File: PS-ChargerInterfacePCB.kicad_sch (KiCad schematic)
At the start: 17 parts, among them J2 LV_Elcon_Connector, J4 PeripheralCAN, J5 Estop 2, J6 Estop 3

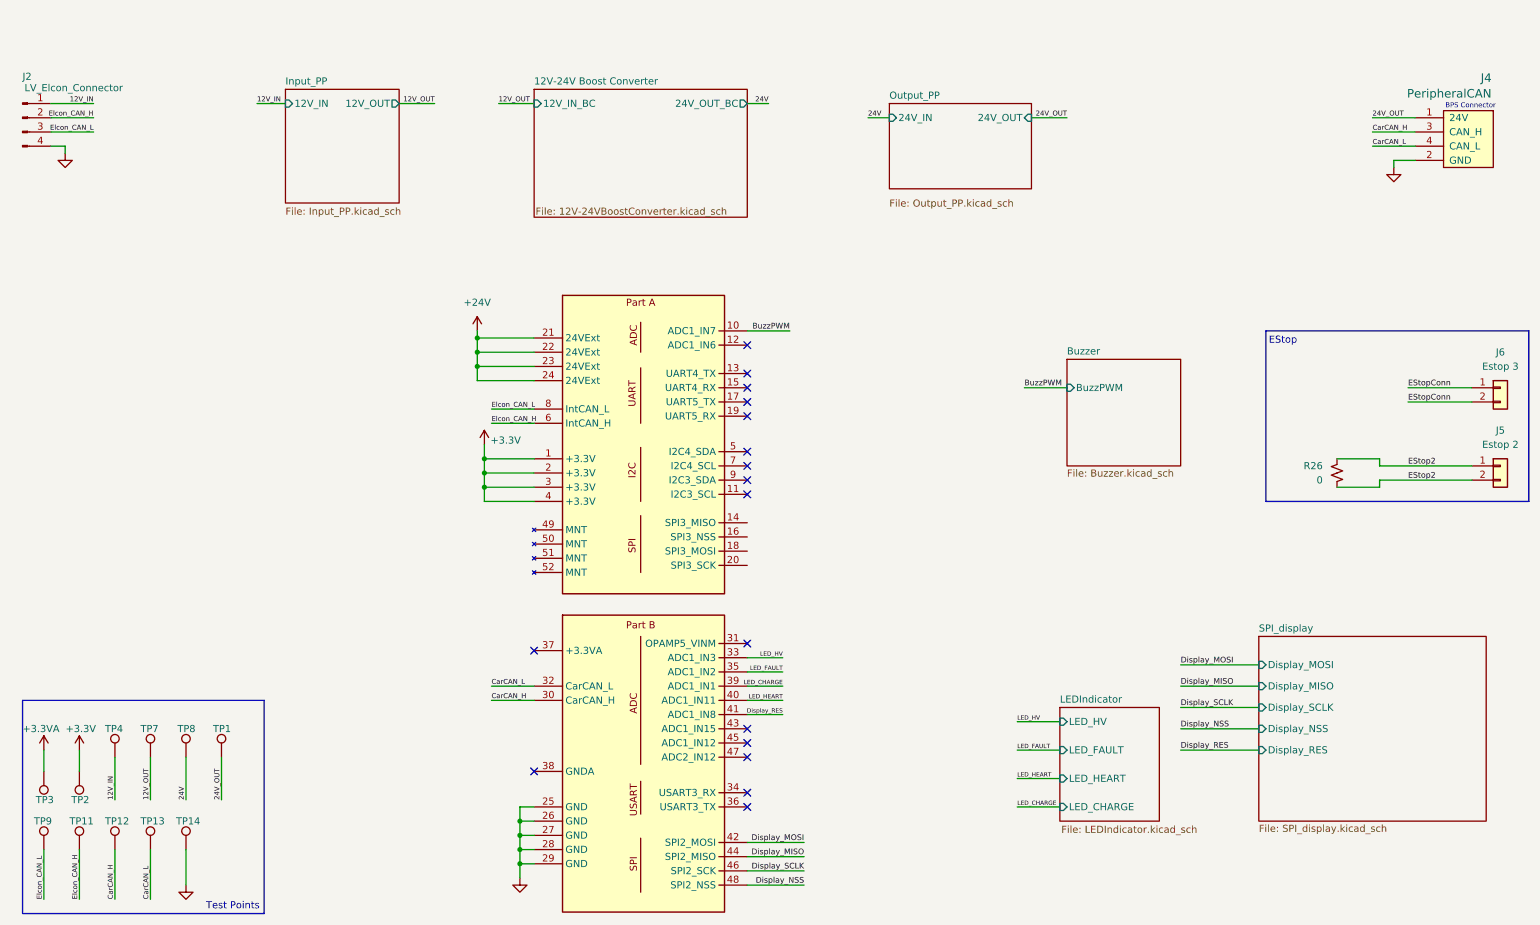
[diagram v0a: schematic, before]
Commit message: revA4
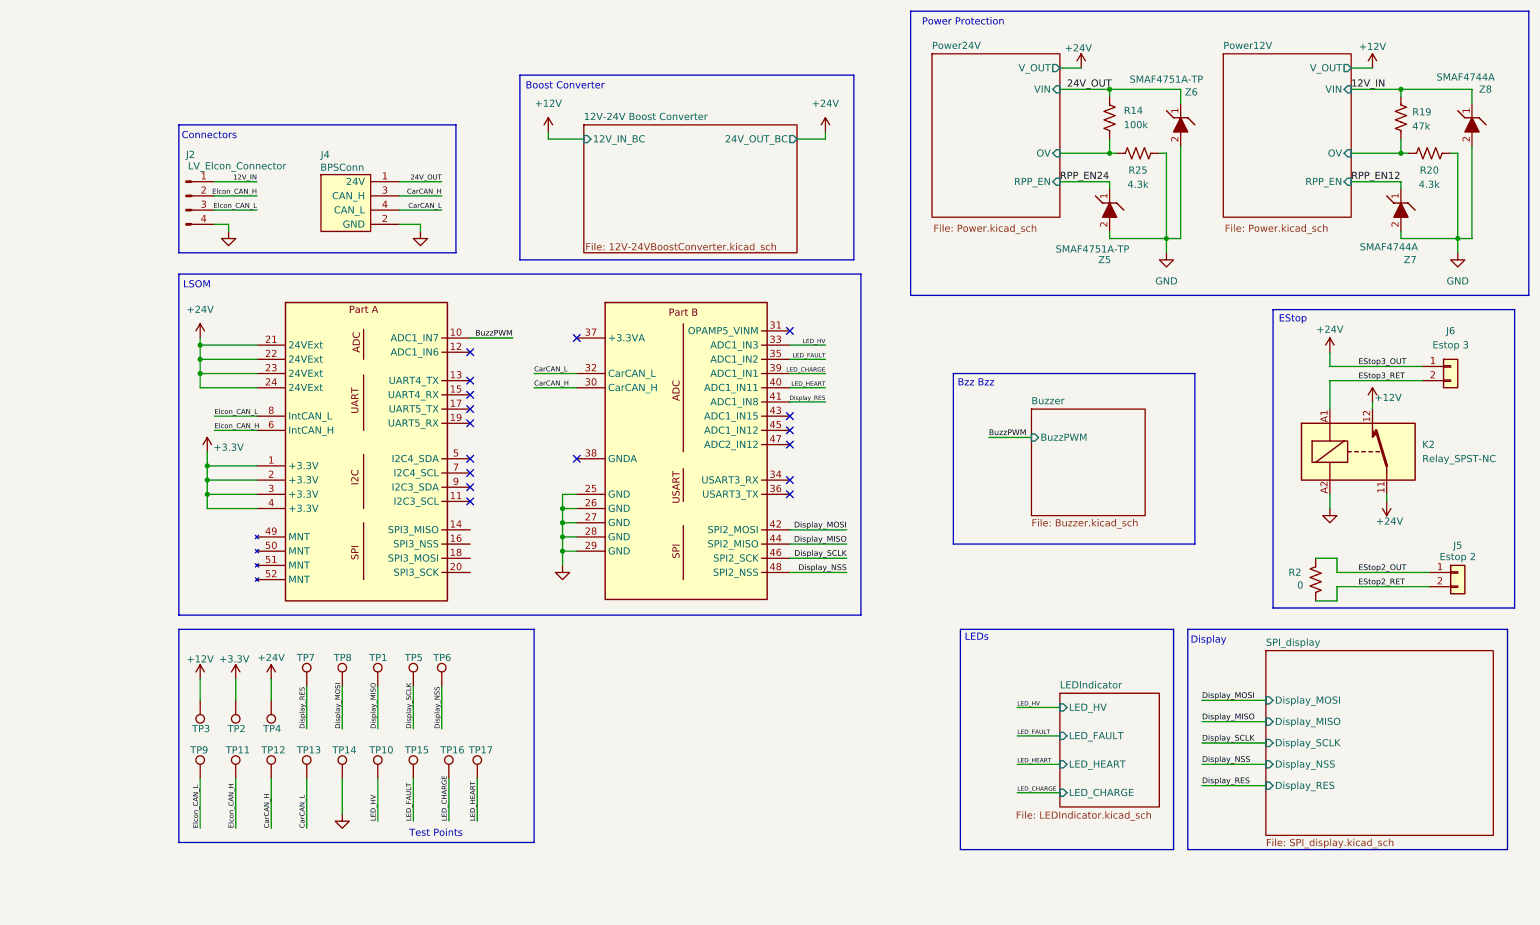
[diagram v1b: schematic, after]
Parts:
- removed R26: 0, symbol Device:R_Small_US
- added K2: Relay_SPST-NC, symbol Relay:Relay_SPST-NC
- added R14: 100k, Resistor_SMD:R_0603_1608Metric, symbol Device:R_US
- added R19: 47k, Resistor_SMD:R_0603_1608Metric, symbol Device:R_US
- added R2: 0, symbol Device:R_US
- added R20, R25: 4.3k, Resistor_SMD:R_0603_1608Metric, symbol Device:R_US
- added TP10, TP15, TP16, TP17, TP5, TP6: TestPoint, symbol Connector:TestPoint
- added Z5, Z6: SMAF4751A-TP, UTSVT_Passives:SODFL5026X125N, symbol UTSVT_Power:SMAF4749A-TP
- added Z7, Z8: SMAF4744A, UTSVT_Passives:SODFL5026X125N, symbol UTSVT_Power:SMAF4749A-TP
- J4: value PeripheralCAN -> BPSConn
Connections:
- net 12V_OUT is gone; now on net Display_RES: TP7.1
- net 24V is gone; now on net Display_MOSI: TP8.1
- net +24V: now also J6.1 (Pin_1), TP4.1, K2.11
- net 12V_IN: now also R19.1, Z8.1 (K); no longer TP4.1
- net 24V_OUT: now also R14.1, Z6.1 (K); no longer TP1.1
- net Display_MISO: now also TP1.1
- net Display_NSS: now also TP6.1
- net Display_SCLK: now also TP5.1
- net GND: now also K2.A2, R20.2, R25.2, Z5.2 (A), Z6.2 (A), Z7.2 (A), Z8.2 (A)
- net LED_CHARGE: now also TP16.1
- net LED_FAULT: now also TP15.1
- net LED_HEART: now also TP17.1
- net LED_HV: now also TP10.1
- net +3.3VA renamed +12V
- net +12V: now also K2.12
- net EStop2 renamed EStop2_OUT
- net EStop2_OUT: now also R2.1; no longer J5.2 (Pin_2)
- net EStopConn renamed EStop3_RET
- net EStop3_RET: now also K2.A1; no longer J6.1 (Pin_1)
- new net EStop2_RET: J5.2 (Pin_2), R2.2
- new net Power12V/OV: R19.2, R20.1
- new net Power24V/OV: R14.2, R25.1
- new net RPP_EN12: Z7.1 (K)
- new net RPP_EN24: Z5.1 (K)
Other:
- removed sheet Input_PP
- removed sheet Output_PP
- added sheet Power12V (Power.kicad_sch)
- added sheet Power24V (Power.kicad_sch)
- note added: "Boost Converter"
- note added: "Bzz Bzz"
- note added: "Connectors"
- note added: "Display"
- note added: "LEDs"
- note added: "LSOM"
- note added: "Power Protection"
- note removed: "BPS Connector"
- moved on the sheet: J2, J4, J5, J6, TP1, TP11, TP12, TP13, TP14, TP2, TP3, TP4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
